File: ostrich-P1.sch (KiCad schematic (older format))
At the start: 6 parts

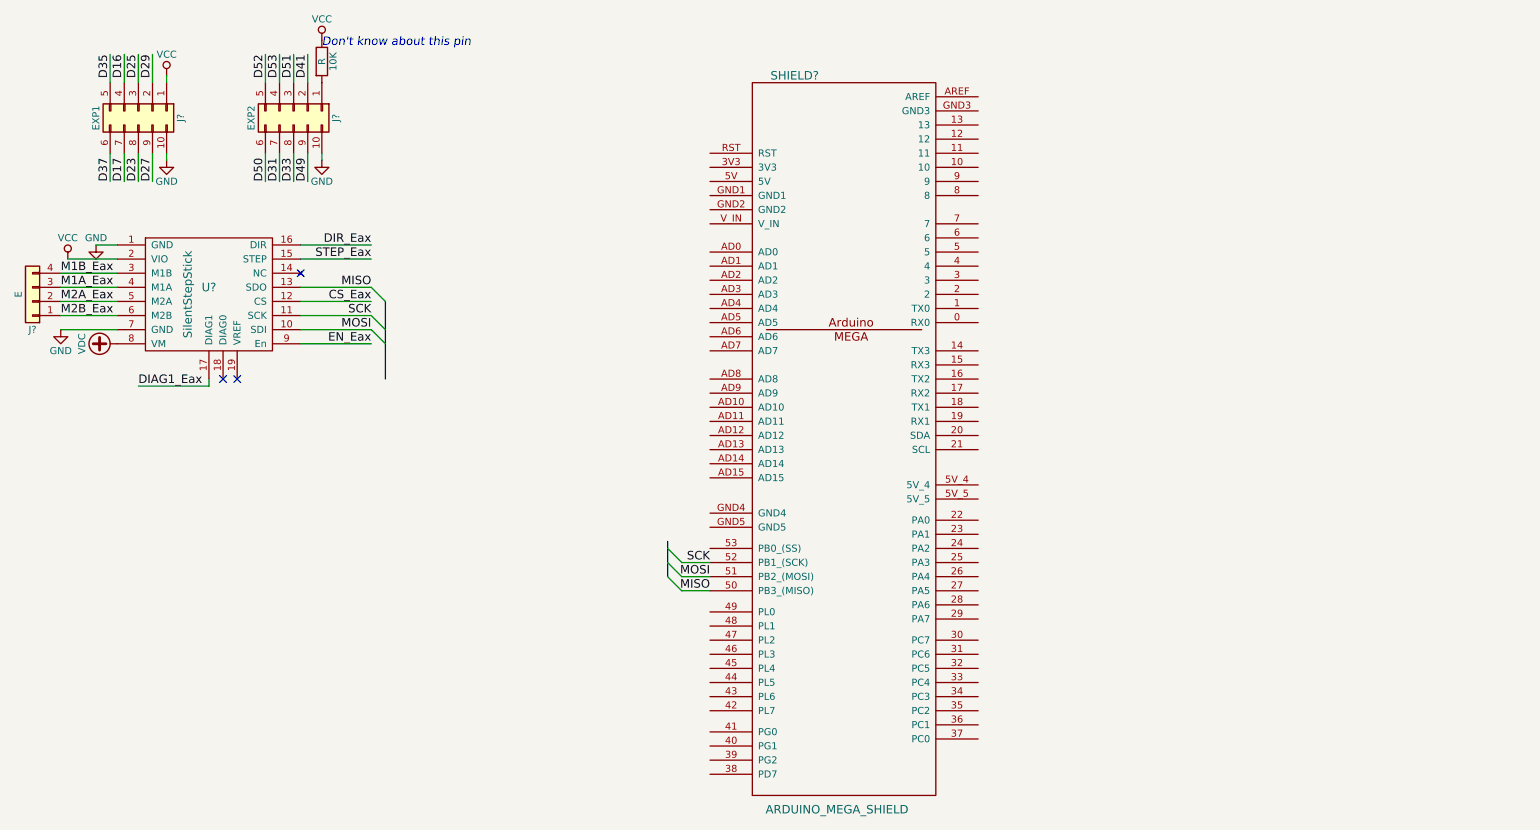
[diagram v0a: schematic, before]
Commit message: Brownout detector done
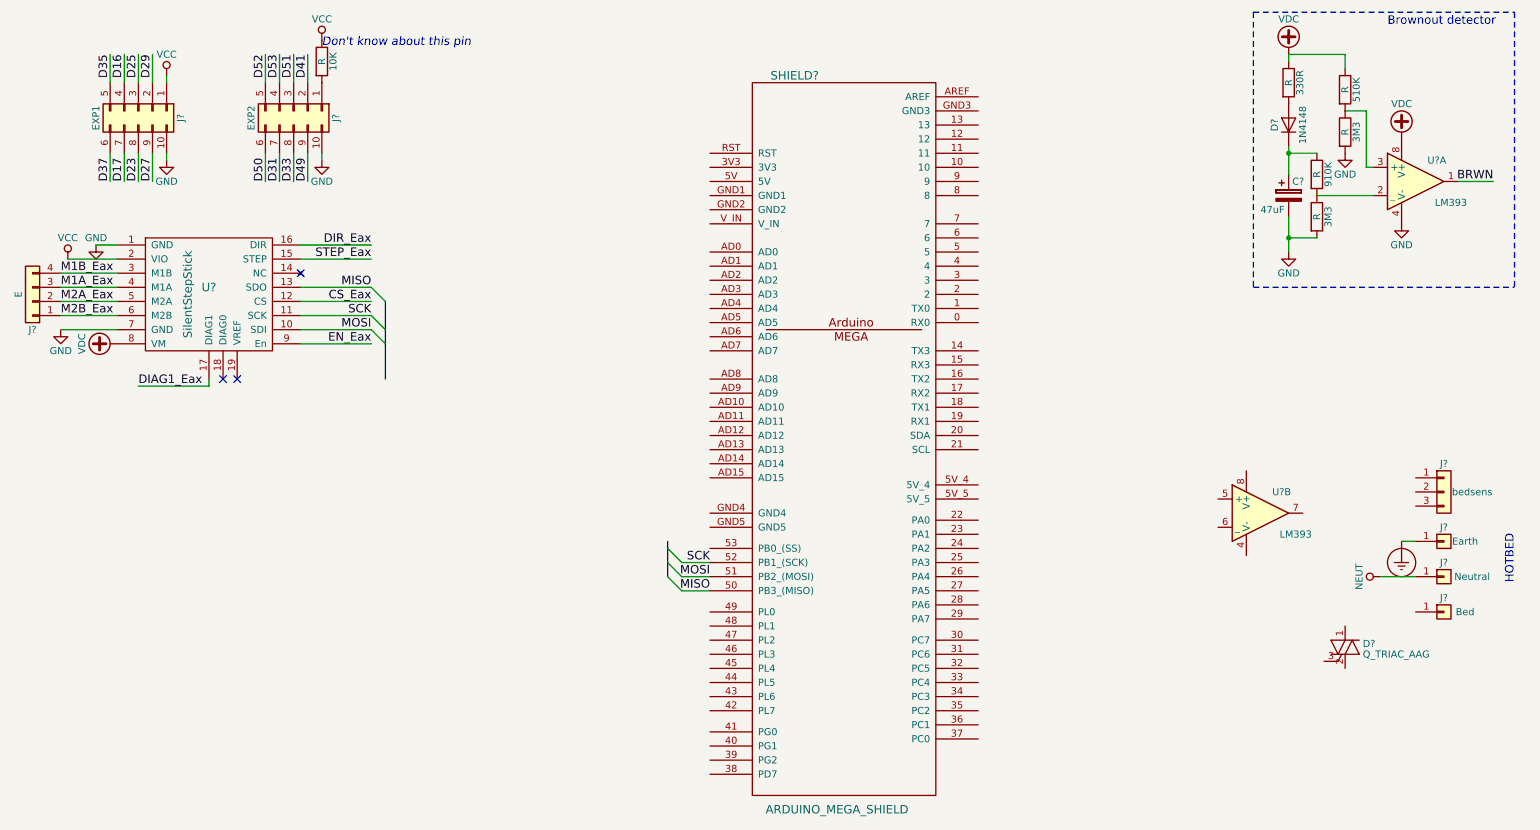
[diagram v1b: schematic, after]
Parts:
- added 330R, 3M3 (x2), 510K, 910K: R, symbol R
- added C?: 47uF, symbol CP
- added D?: 1N4148, symbol D
- added D?: Q_TRIAC_AAG, symbol Q_TRIAC_AAG
- added J?: bedsens, symbol Conn_01x03
- added J?: Earth, symbol Conn_01x01
- added J?: Neutral, symbol Conn_01x01
- added J?: Bed, symbol Conn_01x01
- added U? (x2): LM393, symbol LM393
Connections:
- net GND: now also 3M3.2, 3M3.2, C?.2, U?.4 (V-)
- net VDC: now also 330R.1, 510K.1, U?.8 (V+)
- new net: 910K.1, C?.1, D?.1 (K)
- new net: 330R.2, D?.2 (A)
- new net: 3M3.1, 910K.2, U?.2 (_)
- new net: 3M3.1, 510K.2, U?.3 (+)
- new net BRWN: U?.1
- new net Earth_Protective: J?.1 (Pin_1)
- new net NEUT: J?.1 (Pin_1)
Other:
- note added: "Brownout detector"
- note added: "HOTBED"
